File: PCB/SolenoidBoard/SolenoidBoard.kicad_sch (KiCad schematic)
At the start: 28 parts, among them IC1 NJW4132U2-B-TE2, J1 XT30, J2 Con_45V, J3 Con_45V, J4 Conn_01x02, J5 Con_GND, J6 Con_GND, J7 Conn_01x03, Q1 SSM6J808RLF, Q2 TPH11006NL,LQ_S, U1 TLP293, U2 TLP293

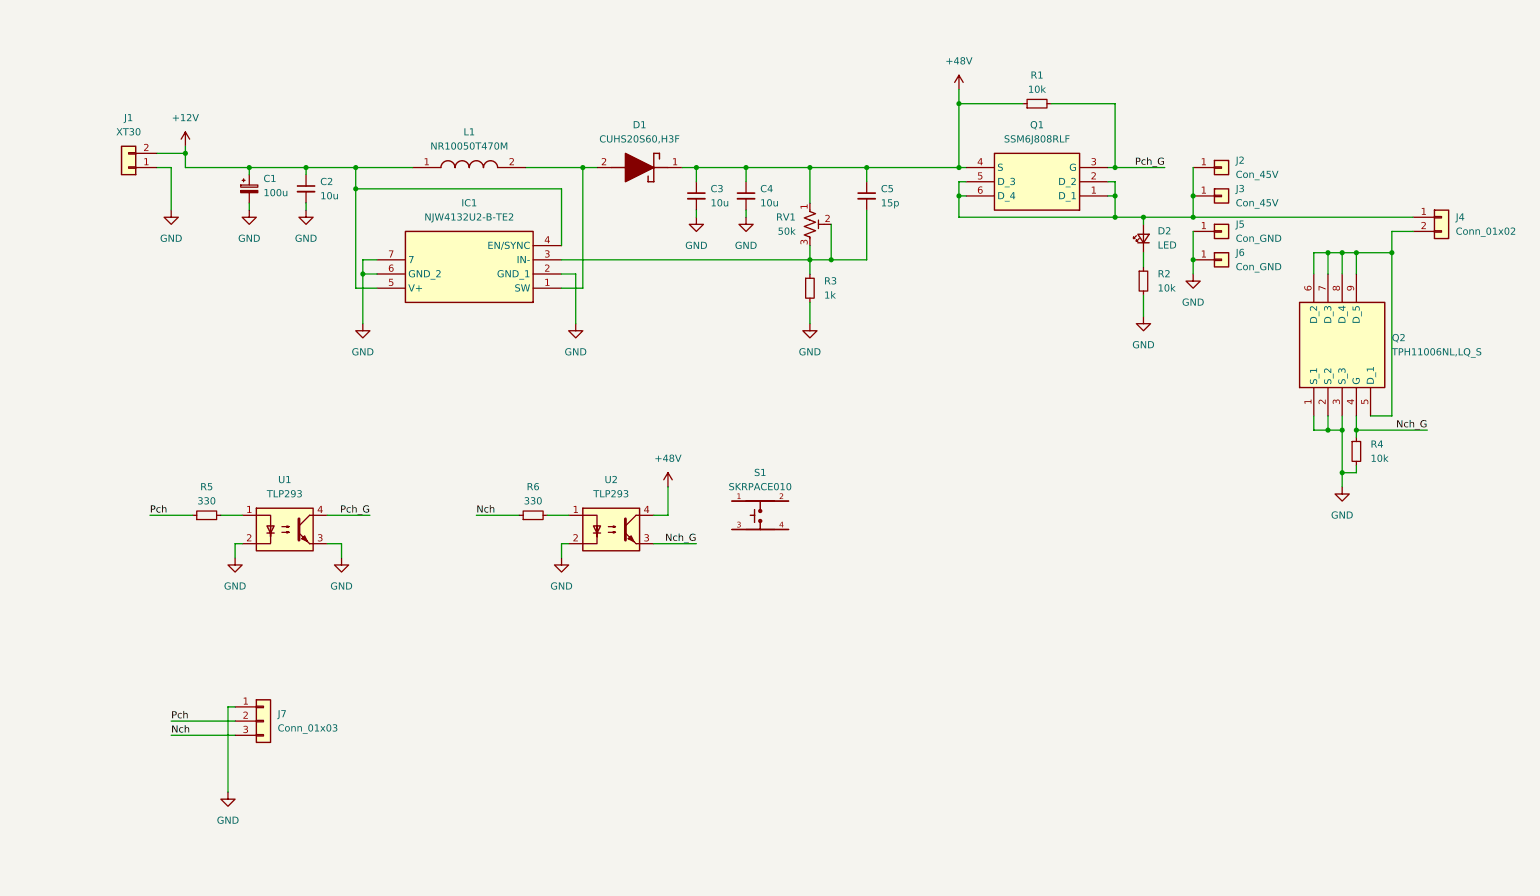
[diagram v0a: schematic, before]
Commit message: 回路図完成
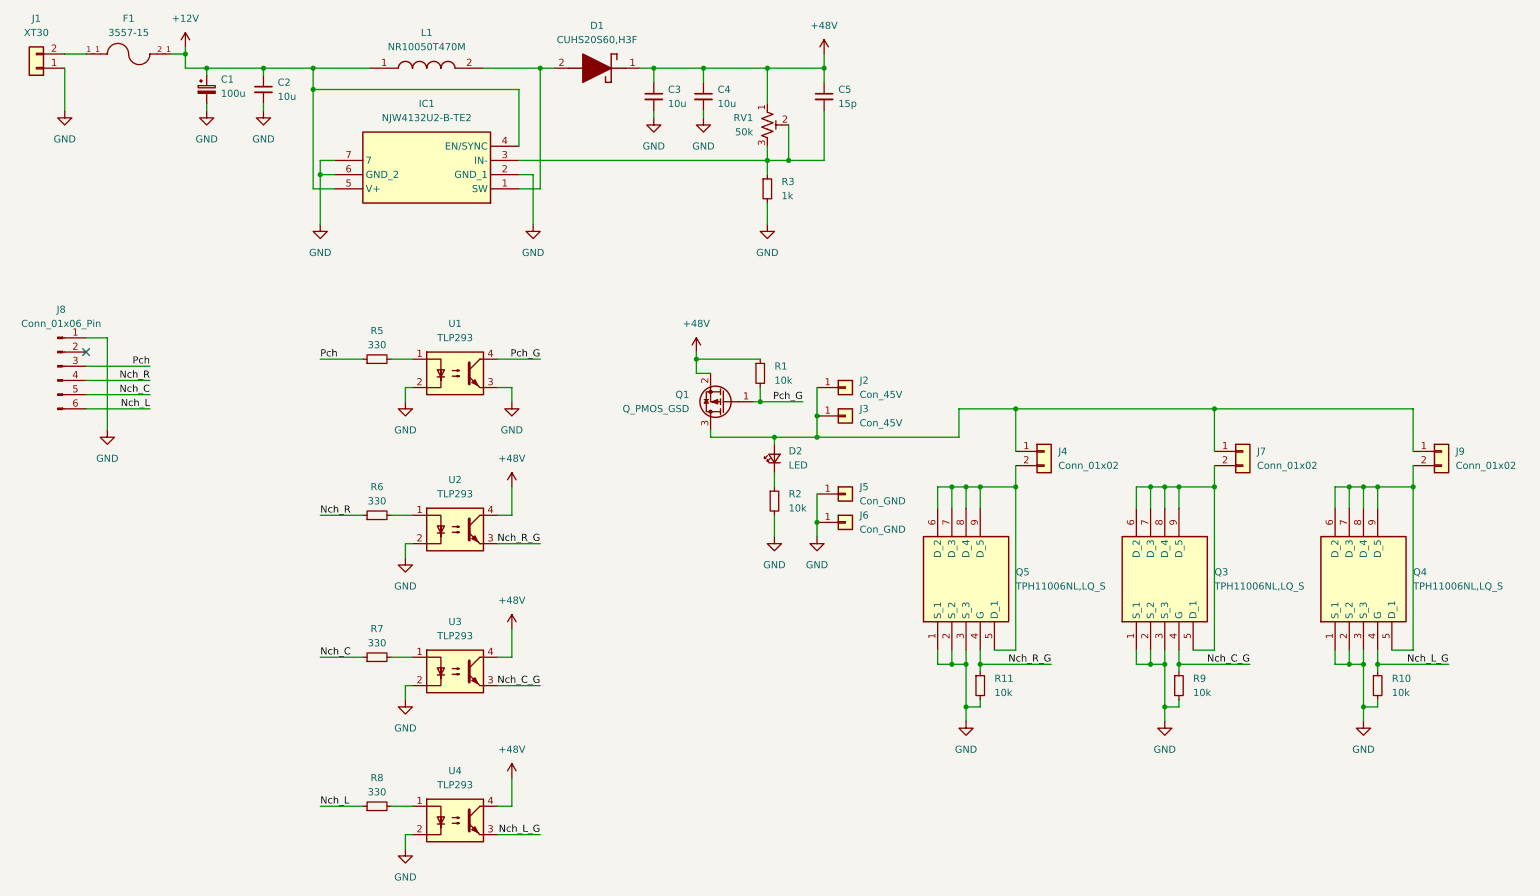
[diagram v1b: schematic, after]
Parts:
- removed J7: Conn_01x03, Connector_JST:JST_PH_S3B-PH-K_1x03_P2.00mm_Horizontal, symbol Connector_Generic:Conn_01x03
- removed Q1: SSM6J808RLF, SSM6J808RLF:SSM6J808RLF, symbol SSM6J808RLF:SSM6J808RLF
- removed Q2: TPH11006NL,LQ_S, TPH11006NL,LQ_S:TPH11006NLLQS, symbol TPH11006NL_LQ_S:TPH11006NL,LQ_S
- removed R4: 10k, Resistor_SMD:R_0603_1608Metric, symbol Device:R_Small
- removed S1: SKRPACE010, SKRPACE010:SW_SKRPACE010, symbol SKRPACE010:SKRPACE010
- added F1: 3557-15, 3557-15:FUSE_3557-15, symbol 3557-15:3557-15
- added J7, J9: Conn_01x02, Connector_JST:JST_XA_S02B-XASK-1_1x02_P2.50mm_Horizontal, symbol Connector_Generic:Conn_01x02
- added J8: Conn_01x06_Pin, symbol Connector:Conn_01x06_Pin
- added Q1: Q_PMOS_GSD, Package_TO_SOT_SMD:SOT-23-3, symbol Transistor_FET:Q_PMOS_GSD
- added Q3, Q4, Q5: TPH11006NL,LQ_S, SOP Advance:SOP Advance, symbol TPH11006NL_LQ_S:TPH11006NL,LQ_S
- added R10, R11, R9: 10k, Resistor_SMD:R_0603_1608Metric, symbol Device:R_Small
- added R7, R8: 330, Resistor_SMD:R_0603_1608Metric, symbol Device:R_Small
- added U3, U4: TLP293, Package_SO:SOIC-4_4.55x2.6mm_P1.27mm, symbol Isolator:TLP293
- D1: footprint CUHS20S60,H3F:CUHS20S60H3F -> Diode_SMD:D_SOD-323_HandSoldering
- IC1: footprint NJW4132U2-B-TE2:NJW4132U2BTE2 -> Package_TO_SOT_SMD:SOT-89-5_Handsoldering
- L1: footprint NR10050T470M:NR10050T470M -> Inductor_SMD:L_10.4x10.4_H4.8
- RV1: footprint TC33X:TC33X2503E -> Potentiometer_SMD:Potentiometer_Bourns_TC33X_Vertical
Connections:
- net +12V: now also F1.2_1, F1.2_2; no longer J1.2 (Pin_2)
- net +48V: now also Q1.2 (S), U3.4, U4.4
- net GND: now also J8.1 (Pin_1), Q3.1 (S_1), Q3.2 (S_2), Q3.3 (S_3), Q4.1 (S_1), Q4.2 (S_2), Q4.3 (S_3), Q5.1 (S_1), Q5.2 (S_2), Q5.3 (S_3), R10.2, R11.2, R9.2, U3.2, U4.2
- net Pch: now also J8.3 (Pin_3)
- net Pch_G: now also Q1.1 (G)
- net at D2.2 (A), J2.1 (Pin_1), J3.1 (Pin_1)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: now also J7.1 (Pin_1), J9.1 (Pin_1), Q1.3 (D)
- net at J4.2 (Pin_2): now also Q5.5 (D_1), Q5.6 (D_2), Q5.7 (D_3), Q5.8 (D_4), Q5.9 (D_5)
- net Nch renamed Nch_R
- net Nch_R: now also J8.4 (Pin_4)
- net Nch_G renamed Nch_R_G
- net Nch_R_G: now also Q5.4 (G), R11.1
- new net: R7.2, U3.1
- new net: F1.1_1, F1.1_2, J1.2 (Pin_2)
- new net: J9.2 (Pin_2), Q4.5 (D_1), Q4.6 (D_2), Q4.7 (D_3), Q4.8 (D_4), Q4.9 (D_5)
- new net: J7.2 (Pin_2), Q3.5 (D_1), Q3.6 (D_2), Q3.7 (D_3), Q3.8 (D_4), Q3.9 (D_5)
- new net: R8.2, U4.1
- new net Nch_C: J8.5 (Pin_5), R7.1
- new net Nch_C_G: Q3.4 (G), R9.1, U3.3
- new net Nch_L: J8.6 (Pin_6), R8.1
- new net Nch_L_G: Q4.4 (G), R10.1, U4.3
- no-connect marks 0 -> 1
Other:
- moved on the sheet: C1, C2, C3, C4, C5, D1, D2, IC1, J1, J2, J3, J4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
